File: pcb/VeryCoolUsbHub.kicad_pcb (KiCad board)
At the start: 4 copper layers, 84.8 x 58.4 mm, 56 parts, among them U1 HD3SS3220RNHR, U2 HD3SS3220RNHR, X1 X322525MSB4SI, X2 X322525MSB4SI

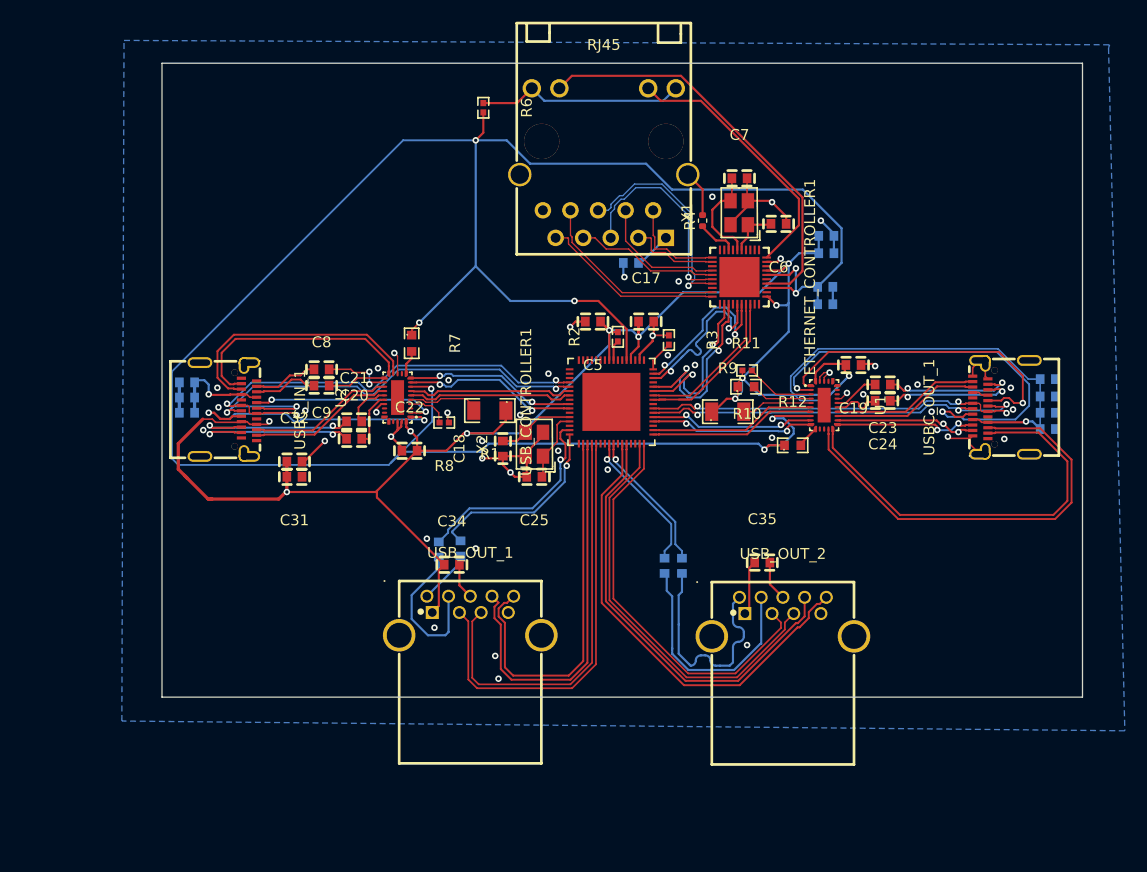
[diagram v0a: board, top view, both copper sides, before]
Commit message: LETSGO THIS GONNA BE THE LAST TIME I ROUTE
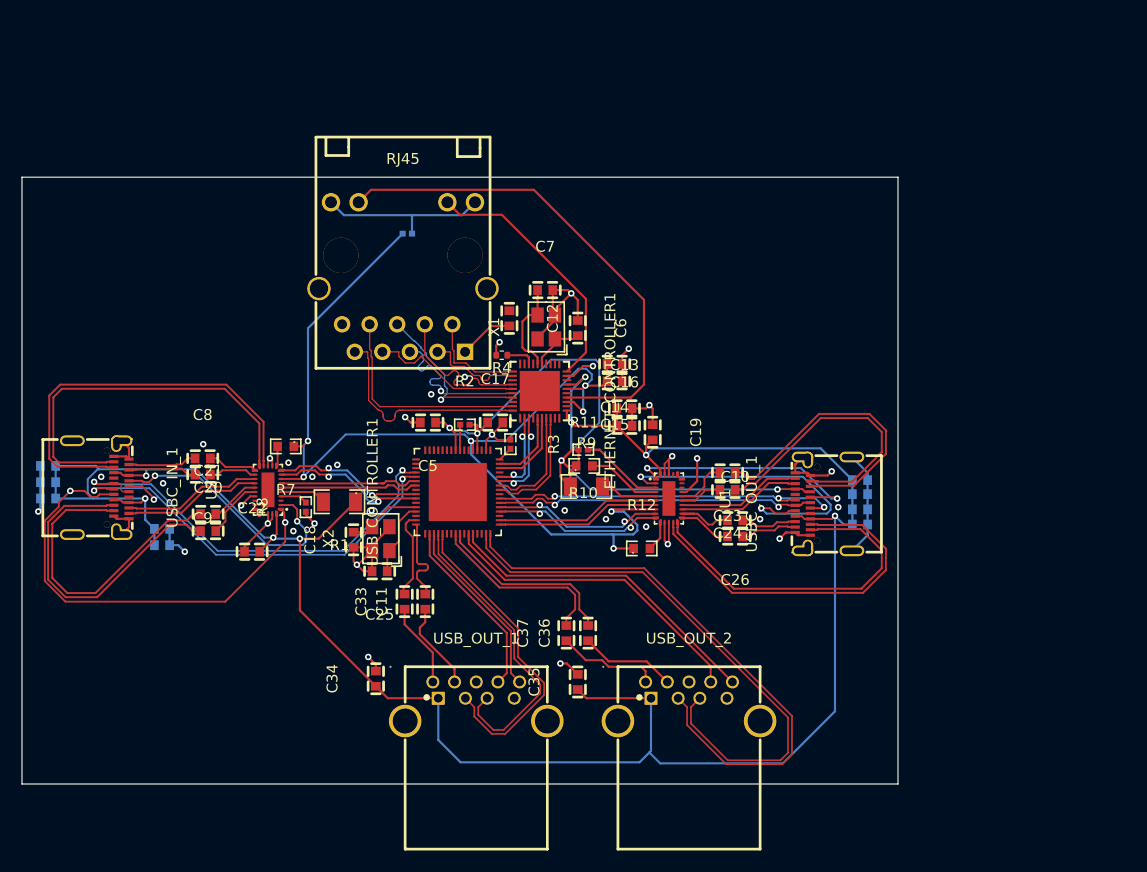
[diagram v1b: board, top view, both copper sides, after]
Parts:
- added C10: CC0603KRX7R9BB104, EasyEDA:C0603, F.Cu at (230.7, 60.8)
- added C26: CC0603KRX7R9BB104, EasyEDA:C0603, F.Cu at (230.7, 62.3)
- C11, C12, C13, C14, C15, C16, C33, C36, C37: moved to F.Cu
- C31, C32, R6: moved to B.Cu
- moved C16 25.5 mm to (220.5, 52.1)
- moved C13 23.5 mm to (220.5, 50.5)
- moved C31 22.7 mm to (167.4, 57.3), turned to 0 degrees
- moved C32 22.7 mm to (167.4, 55.8), turned to 180 degrees
- moved R4 22.3 mm to (209.2, 45.6), turned to 180 degrees
- moved RJ45 21.3 mm to (200.1, 38.4)
- moved ETHERNET_CONTROLLER1 21.2 mm to (212.7, 48.9)
- moved C6 20.8 mm to (216.2, 43.1), turned to -90 degrees
- moved C14 20.7 mm to (219.6, 46.4)
- moved C15 20.7 mm to (219.6, 48.0)
- moved X1 20.7 mm to (213.3, 43.0)
- moved C7 20.7 mm to (213.2, 39.6)
- moved C35 20.2 mm to (216.2, 75.7), turned to 90 degrees
- moved C4 19.6 mm to (242.2, 57.1)
- moved C19 19.5 mm to (223.1, 52.7), turned to -90 degrees
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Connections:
- C11 pad 2: /TXN1 -> /TXP1
- C20 pad 1: /USBC_IN_TXP2 -> /USBC_IN_TXN2
- C21 pad 1: /USBC_IN_TXN2 -> /USBC_IN_TXP2
- C23 pad 1: /USBC_OUT_TXP2 -> /USBC_OUT_TXN2
- C24 pad 1: /USBC_OUT_TXN2 -> /USBC_OUT_TXP2
- C33 pad 2: /TXP1 -> /TXN1
- C35 pad 1: Net-(USB_OUT_2-Vbus) -> VBUS
- C36 pad 2: /TXN2 -> /TXP2
- C37 pad 2: /TXP2 -> /TXN2
- C8 pad 1: /USBC_IN_TXN1 -> /USBC_IN_TXP1
- C9 pad 2: /USBC_IN_TXP1 -> /USBC_IN_TXN1
- ETHERNET_CONTROLLER1 pad 12: /TXN4 -> /TXP4
- ETHERNET_CONTROLLER1 pad 13: /TXP4 -> /TXN4
- ETHERNET_CONTROLLER1 pad 15: /RXN4 -> /RXP4
- ETHERNET_CONTROLLER1 pad 16: /RXP4 -> /RXN4
- U1 pad 16: /USBC_OUT_TXN1 -> Net-(U1-TX1n)
- U1 pad 17: /USBC_OUT_TXP1 -> Net-(U1-TX1p)
- USB_OUT_1 pad 5: /RXN1 -> /RXP1
- USB_OUT_1 pad 6: /RXP1 -> /RXN1
- USB_OUT_2 pad 1: Net-(USB_OUT_2-Vbus) -> VBUS
- USB_OUT_2 pad 5: /RXN2 -> /RXP2
- USB_OUT_2 pad 6: /RXP2 -> /RXN2
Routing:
- net /V3.3: track 220.7 -> 104.0 mm, vias 8 -> 7
- net VBUS: track 217.5 -> 285.5 mm, vias 13 -> 12
- net GND: track 75.5 -> 101.7 mm, vias 46 -> 37
- net /RXP1: track 36.6 -> 16.9 mm
- net /RXN1: track 35.6 -> 16.9 mm
- net /USBC_IN_CC2: track 25.5 -> 42.0 mm
- net /DN2: track 37.1 -> 53.3 mm
- net /USBC_OUT_TXN2: track 12.3 -> 27.6 mm, vias 2 -> 0
- net /USBC_OUT_TXP2: track 12.5 -> 26.3 mm, vias 2 -> 0
- net /DP2: track 38.3 -> 52.1 mm
- net /USBC_IN_RXP1: track 22.2 -> 35.8 mm
- net /RXN2: track 43.0 -> 29.3 mm
- net /USBC_IN_TXN2: track 16.1 -> 29.7 mm, vias 2 -> 0
- net /USBC_IN_RXN1: track 24.1 -> 37.7 mm
- net Net-(USB_OUT_2-StdA_SSTX-): track 21.9 -> 8.87 mm
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- removed copper zone on B.Cu, net GND
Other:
- board size 84.8 x 58.4 mm -> 80.7 x 55.9 mm
